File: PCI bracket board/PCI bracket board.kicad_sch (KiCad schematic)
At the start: 9 parts, among them J3 microphone, J4 line out, J5 speaker in, J6 speaker out, J7 serial

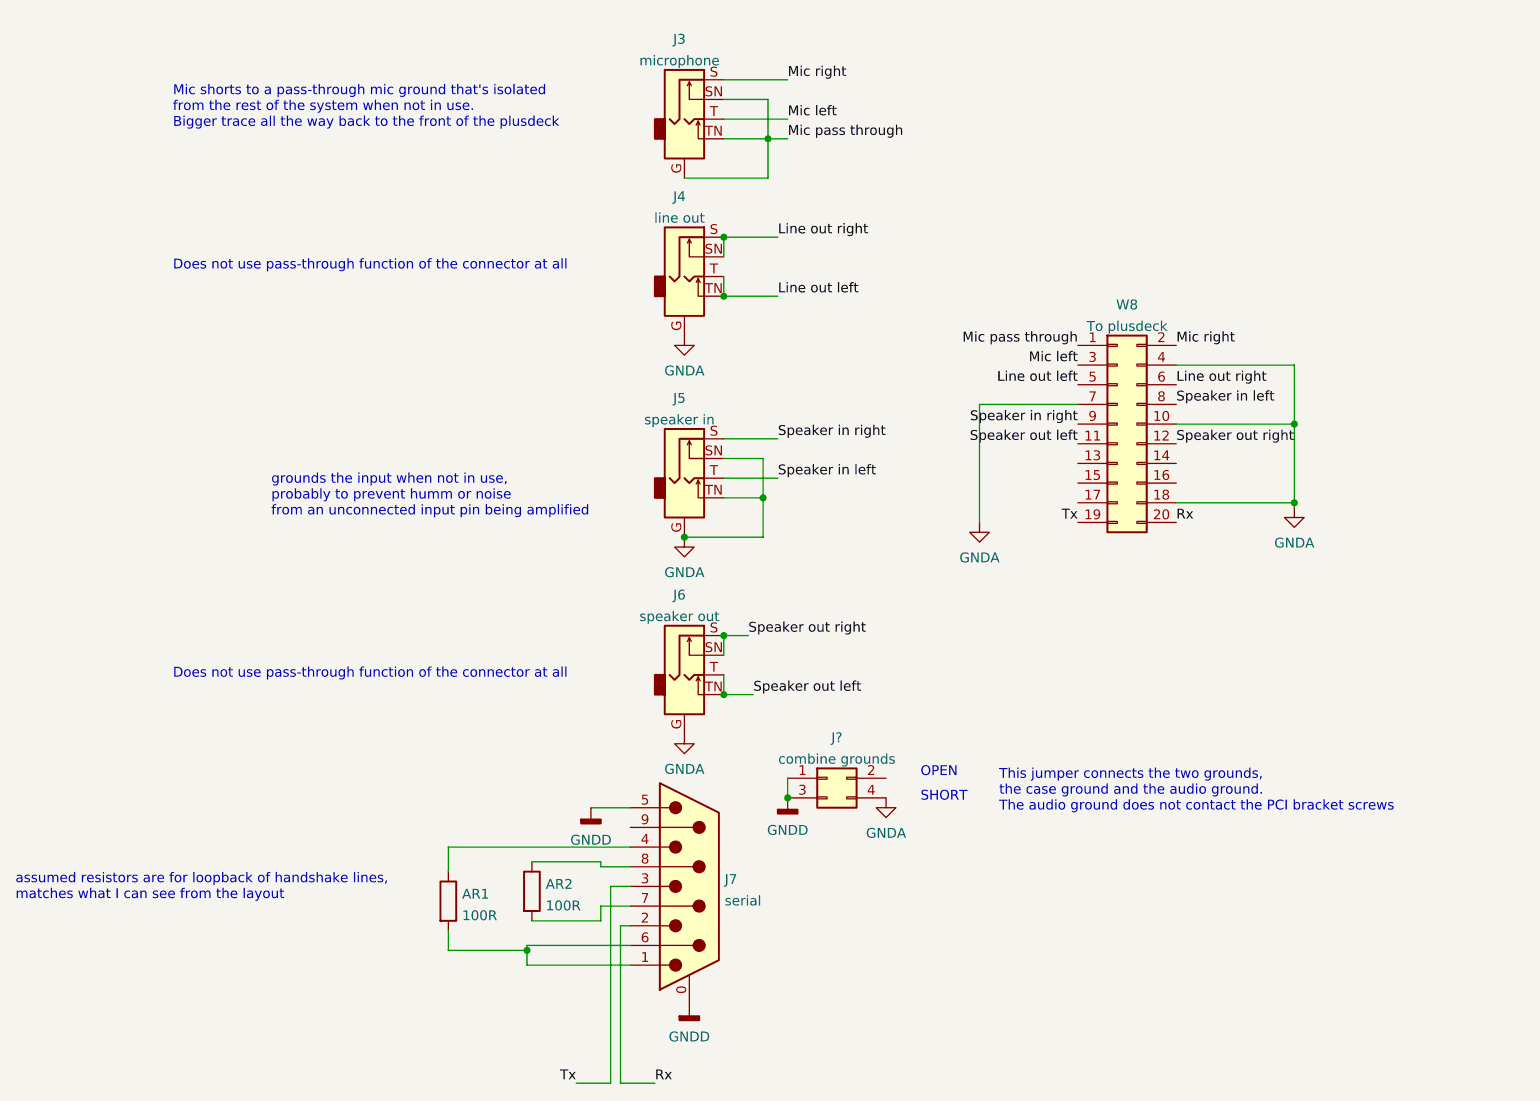
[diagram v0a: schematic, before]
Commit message: added layout
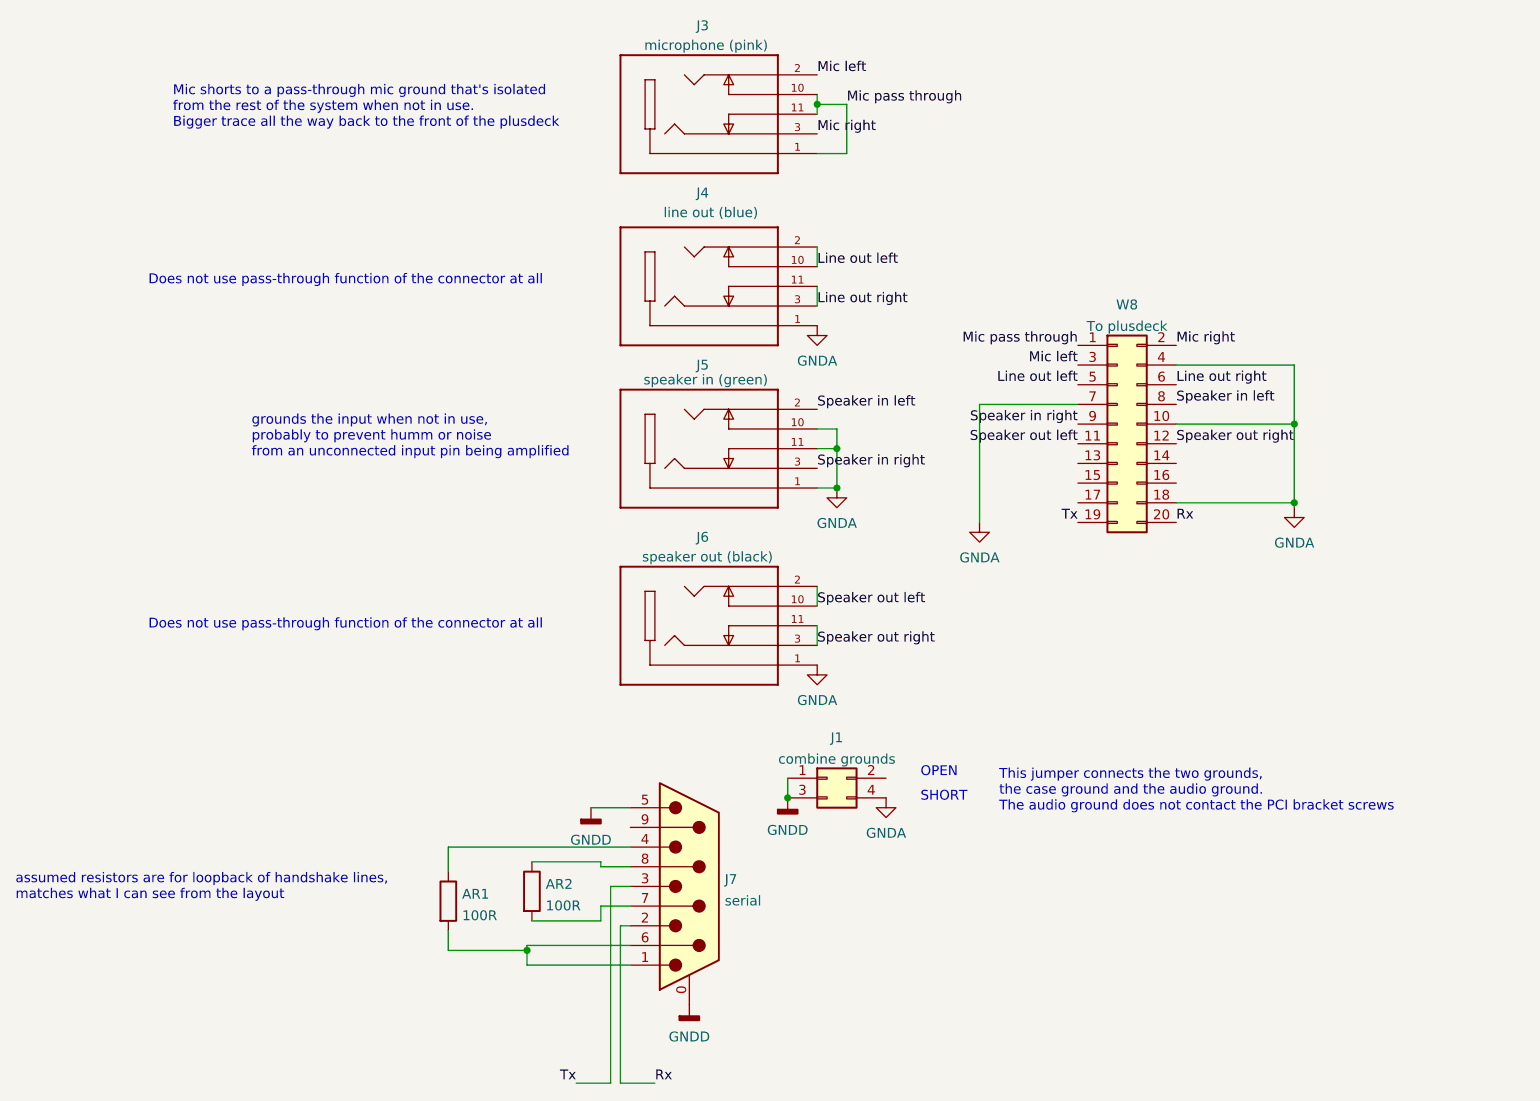
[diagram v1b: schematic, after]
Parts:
- removed J3: microphone, symbol Connector:AudioJack2_Ground_Switch
- removed J4: line out, symbol Connector:AudioJack2_Ground_Switch
- removed J5: speaker in, symbol Connector:AudioJack2_Ground_Switch
- removed J6: speaker out, symbol Connector:AudioJack2_Ground_Switch
- added J3: microphone (pink), Evan's misc parts:CUI_SJ1-3525N, symbol Evan's misc parts:SJ1-3525N
- added J4: line out (blue), Evan's misc parts:CUI_SJ1-3525N, symbol Evan's misc parts:SJ1-3525N
- added J5: speaker in (green), Evan's misc parts:CUI_SJ1-3525N, symbol Evan's misc parts:SJ1-3525N
- added J6: speaker out (black), Evan's misc parts:CUI_SJ1-3525N, symbol Evan's misc parts:SJ1-3525N
- AR1, AR2: footprint (none) -> Resistor_THT:R_Axial_DIN0207_L6.3mm_D2.5mm_P10.16mm_Horizontal
- J1: renamed from J?; footprint (none) -> Connector_PinHeader_2.54mm:PinHeader_2x02_P2.54mm_Vertical
- J7: footprint (none) -> Connector_Dsub:DSUB-9_Male_Horizontal_P2.77x2.84mm_EdgePinOffset7.70mm_Housed_MountingHolesOffset9.12mm
- W8: footprint (none) -> Connector_PinHeader_2.54mm:PinHeader_2x10_P2.54mm_Horizontal
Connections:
- net GNDA: now also J4.1, J5.1, J5.10, J5.11, J6.1
- net Line out left: now also J4.10, J4.2
- net Line out right: now also J4.11, J4.3
- net Mic left: now also J3.2
- net Mic pass through: now also J3.1, J3.10, J3.11
- net Mic right: now also J3.3
- net Speaker in left: now also J5.2
- net Speaker in right: now also J5.3
- net Speaker out left: now also J6.10, J6.2
- net Speaker out right: now also J6.11, J6.3
